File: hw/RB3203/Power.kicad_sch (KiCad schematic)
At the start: 21 parts

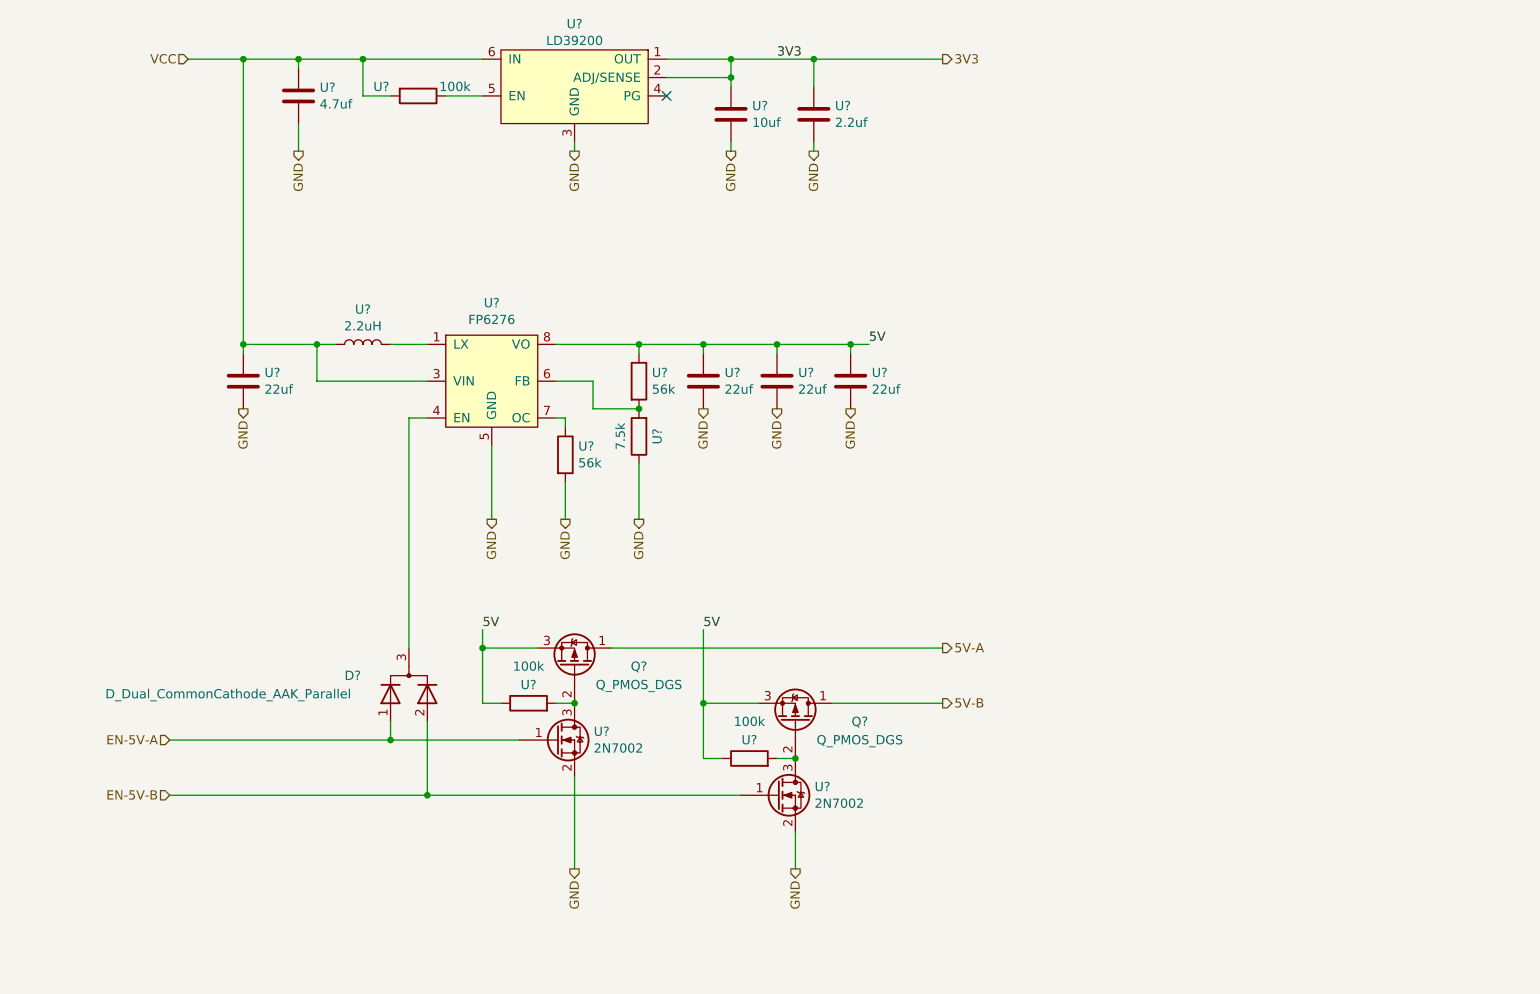
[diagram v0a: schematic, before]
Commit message: Wip
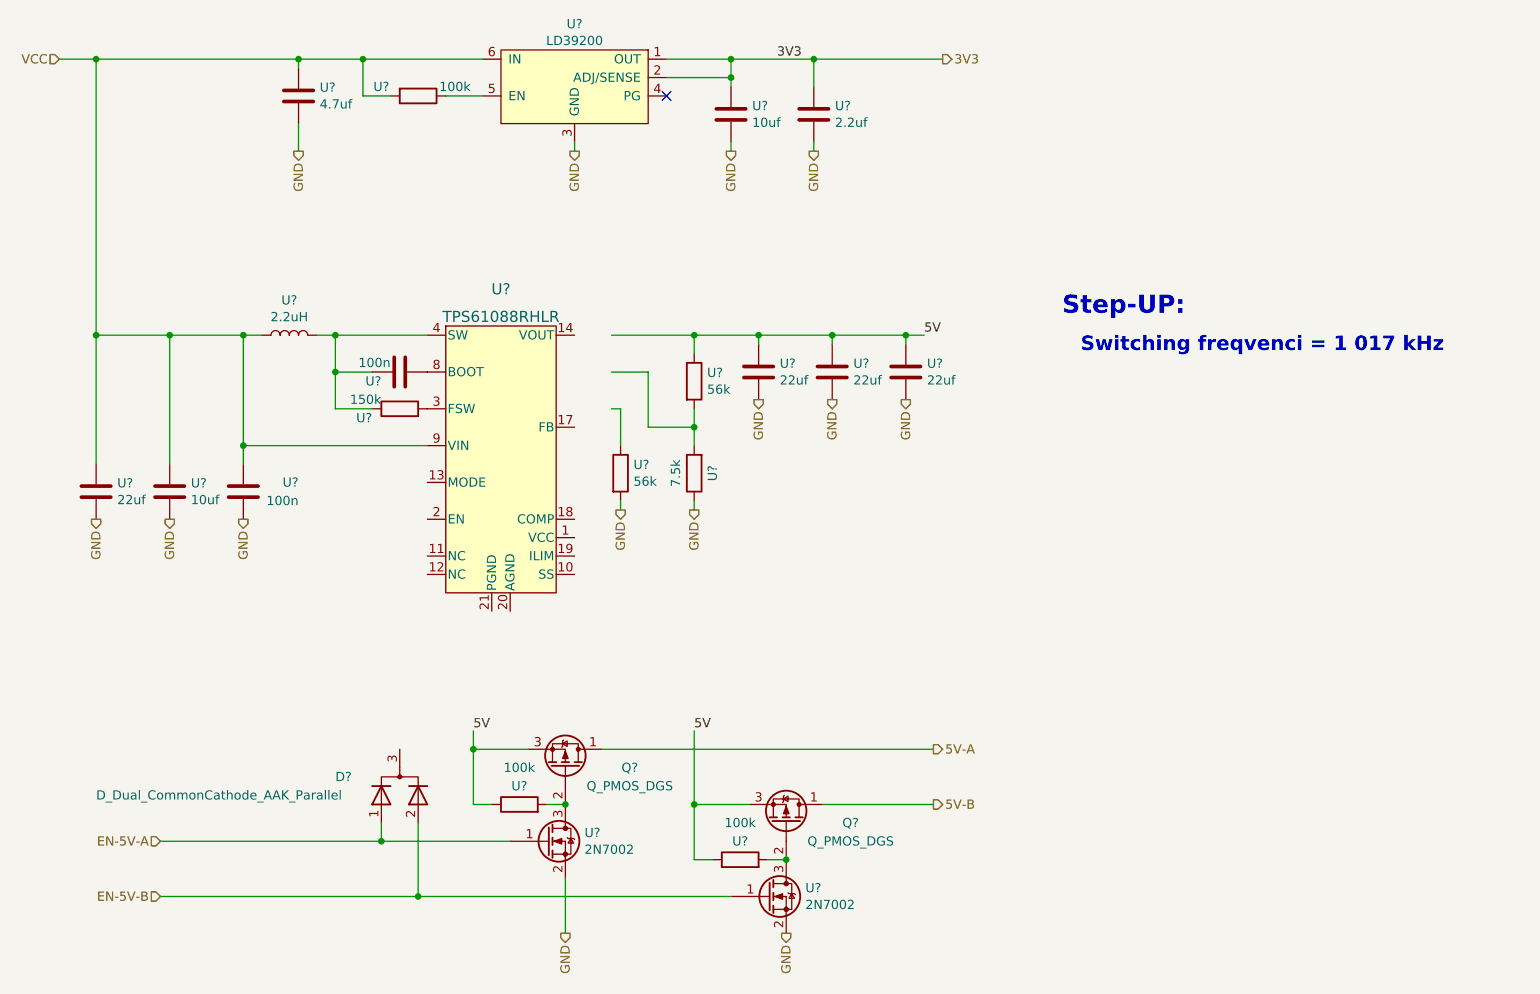
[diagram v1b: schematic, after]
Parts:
- removed U?: FP6276, Package_SO:SOIC-8-1EP_3.9x4.9mm_P1.27mm_EP2.41x3.81mm_ThermalVias, symbol B.B-rescue:FP6276-B.B-rescue-B.B-rescue
- added U? (x2): 100n, Capacitor_SMD:C_0402_1005Metric, symbol B.B-rescue:C-Device-B.B-rescue-B.B-rescue
- added U?: TPS61088RHLR, RHL0020A, symbol Robotarna_KiCad_Library:TPS61088RHLR
- added U?: 150k, Resistor_SMD:R_0402_1005Metric, symbol B.B-rescue:R-Device-B.B-rescue-B.B-rescue
- added U?: 10uf, Capacitor_SMD:C_0805_2012Metric, symbol B.B-rescue:C-Device-B.B-rescue-B.B-rescue
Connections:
- net GND: now also U?.2, U?.2
- net VCC: now also U?.1, U?.1, U?.9 (VIN)
- net LX renamed SW
- net SW: now also U?.1, U?.1, U?.4 (SW), U?.5 (SW), U?.6 (SW), U?.7 (SW)
- new net: U?.2, U?.8 (BOOT)
- new net: U?.14 (VOUT), U?.15 (VOUT), U?.16 (VOUT)
- new net: U?.2, U?.3 (FSW)
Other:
- note added: "Step-UP:"
- note added: "Switching freqvenci = 1 017 kHz"
- moved on the sheet: D?, Q?, U?
